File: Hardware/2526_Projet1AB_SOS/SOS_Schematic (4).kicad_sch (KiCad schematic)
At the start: 40 parts, among them J4 Conn_ST_STDC14, J5 USB_C_Receptacle_USB2.0_14P, SW1 SW_SPDT, U1 BU33SD5WG-TR, U2 STM32L476RGTx, U4 USBLC6-2SC6, Y1 13,56MHz, Y2 8MHz

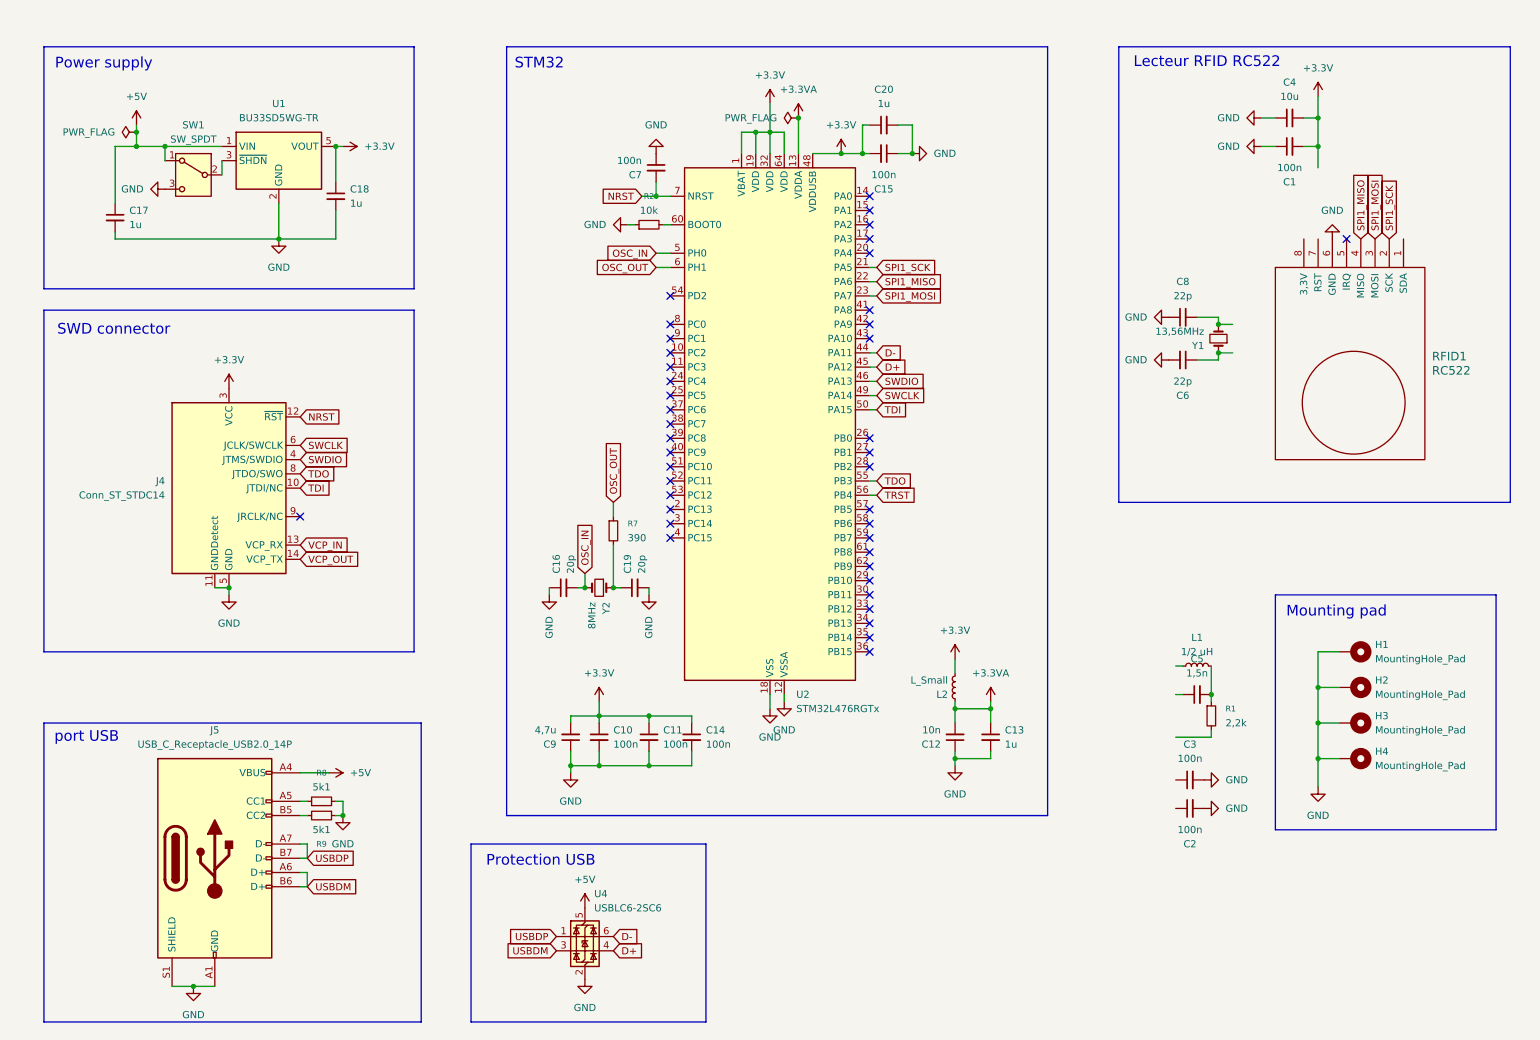
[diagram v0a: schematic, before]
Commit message: schematic v2
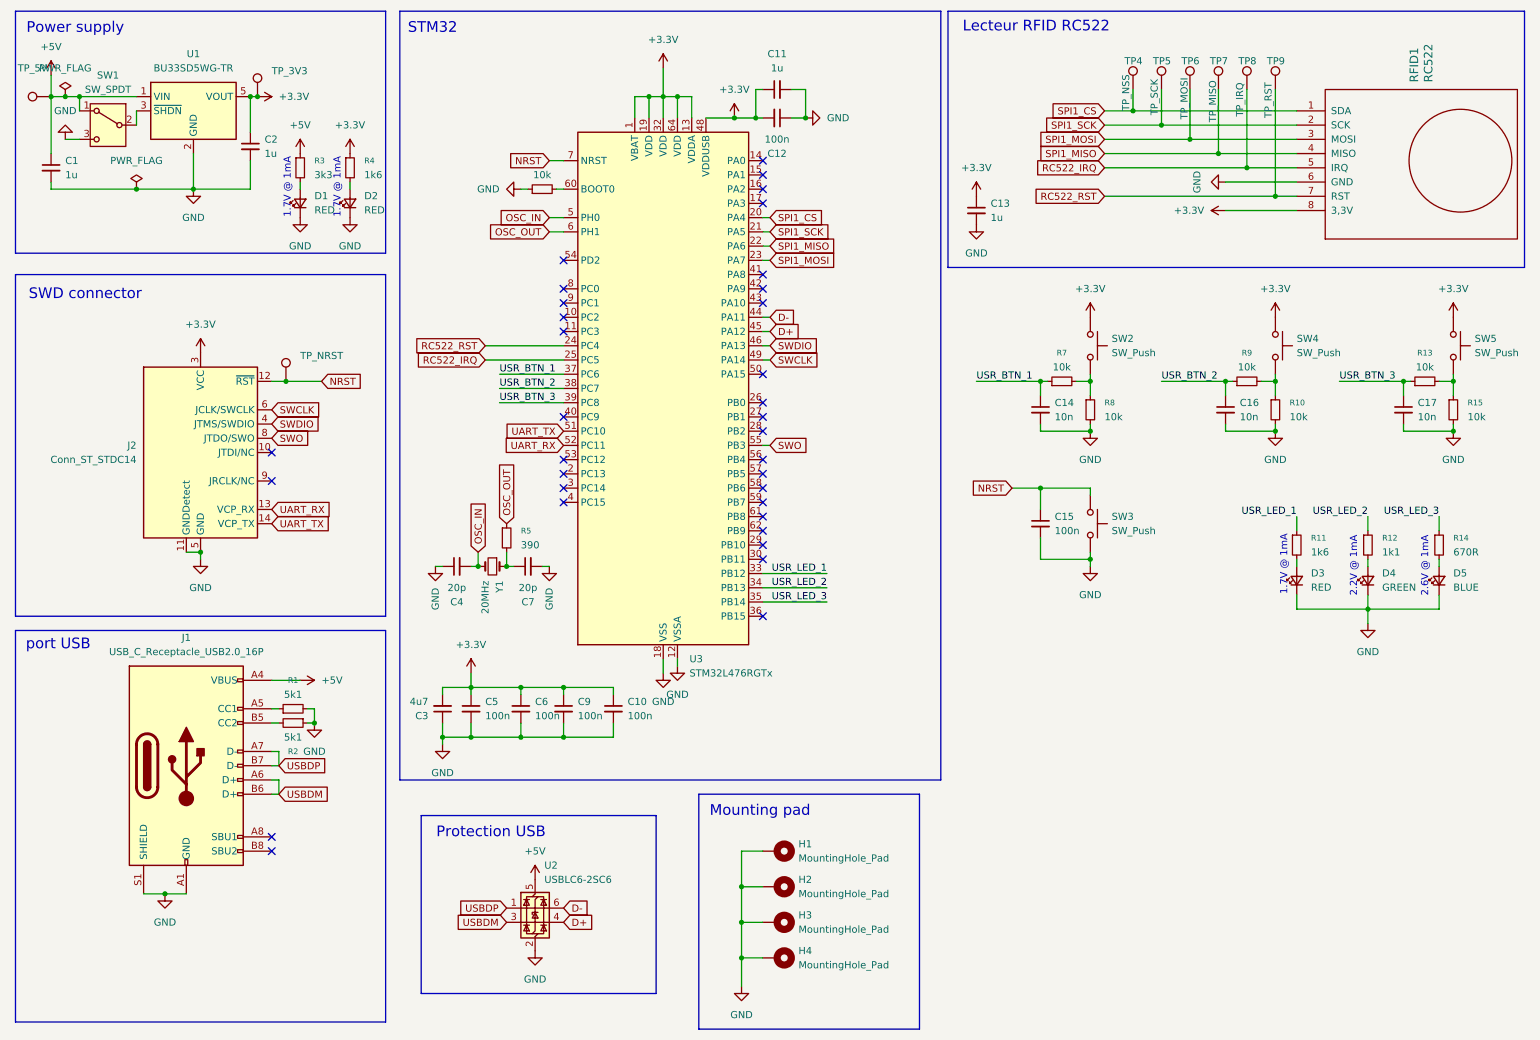
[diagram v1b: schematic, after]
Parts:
- removed C1, C2, C3, C7: 100n, Capacitor_SMD:C_0603_1608Metric_Pad1.08x0.95mm_HandSolder, symbol Device:C_Small
- removed C12: 10n, Capacitor_SMD:C_0603_1608Metric_Pad1.08x0.95mm_HandSolder, symbol Device:C_Small
- removed C4: 10u, Capacitor_SMD:C_0603_1608Metric_Pad1.08x0.95mm_HandSolder, symbol Device:C_Small
- removed C5: 1,5n, Capacitor_SMD:C_0603_1608Metric_Pad1.08x0.95mm_HandSolder, symbol Device:C_Small
- removed C6, C8: 22p, Capacitor_SMD:C_0603_1608Metric_Pad1.08x0.95mm_HandSolder, symbol Device:C_Small
- removed J5: USB_C_Receptacle_USB2.0_14P, symbol Connector:USB_C_Receptacle_USB2.0_14P
- removed L1: 1/2 uH, Inductor_SMD:L_0805_2012Metric_Pad1.05x1.20mm_HandSolder, symbol Device:L_Small
- removed L2: L_Small, Inductor_SMD:L_0805_2012Metric_Pad1.05x1.20mm_HandSolder, symbol Device:L_Small
- removed R1: 2,2k, Resistor_SMD:R_0805_2012Metric_Pad1.20x1.40mm_HandSolder, symbol Device:R_Small
- removed Y1: 13,56MHz, Crystal:Crystal_DS10_D1.0mm_L4.3mm_Vertical, symbol Device:Crystal_Small
- added C10, C15: 100n, Capacitor_SMD:C_0603_1608Metric, symbol Device:C_Small
- added C14, C16, C17: 10n, Capacitor_SMD:C_0603_1608Metric, symbol Device:C_Small
- added D1, D2, D3: RED, LED_SMD:LED_0603_1608Metric, symbol Device:LED_Small
- added D4: GREEN, LED_SMD:LED_0603_1608Metric, symbol Device:LED_Small
- added D5: BLUE, LED_SMD:LED_0603_1608Metric, symbol Device:LED_Small
- added J1: USB_C_Receptacle_USB2.0_16P, symbol Connector:USB_C_Receptacle_USB2.0_16P
- added R10, R13, R15, R7, R8, R9: 10k, Resistor_SMD:R_0603_1608Metric, symbol Device:R_Small
- added R11, R4: 1k6, Resistor_SMD:R_0603_1608Metric, symbol Device:R_Small
- added R12: 1k1, Resistor_SMD:R_0603_1608Metric, symbol Device:R_Small
- added R14: 670R, Resistor_SMD:R_0603_1608Metric, symbol Device:R_Small
- added R3: 3k3, Resistor_SMD:R_0603_1608Metric, symbol Device:R_Small
- added SW2, SW3, SW4, SW5: SW_Push, Button_Switch_SMD:SW_SPST_B3S-1000, symbol Switch:SW_Push
- added TP4: TP_NSS, TestPoint:TestPoint_Pad_D1.0mm, symbol Connector:TestPoint
- added TP5: TP_SCK, TestPoint:TestPoint_Pad_D1.0mm, symbol Connector:TestPoint
- added TP6: TP_MOSI, TestPoint:TestPoint_Pad_D1.0mm, symbol Connector:TestPoint
- added TP7: TP_MISO, TestPoint:TestPoint_Pad_D1.0mm, symbol Connector:TestPoint
- added TP8: TP_IRQ, TestPoint:TestPoint_Pad_D1.0mm, symbol Connector:TestPoint
- added TP9: TP_RST, TestPoint:TestPoint_Pad_D1.0mm, symbol Connector:TestPoint
- added TP_3V3: TP_3V3, TestPoint:TestPoint_Pad_D1.0mm, symbol Connector:TestPoint
- added TP_5V: TP_5V, TestPoint:TestPoint_Pad_D1.0mm, symbol Connector:TestPoint
- added TP_NRST: TP_NRST, TestPoint:TestPoint_Pad_D1.0mm, symbol Connector:TestPoint
- C1: renamed from C17; footprint Capacitor_SMD:C_0603_1608Metric_Pad1.08x0.95mm_HandSolder -> Capacitor_SMD:C_0603_1608Metric
- C11: renamed from C20; footprint Capacitor_SMD:C_0603_1608Metric_Pad1.08x0.95mm_HandSolder -> Capacitor_SMD:C_0603_1608Metric
- C12: renamed from C15; footprint Capacitor_SMD:C_0603_1608Metric_Pad1.08x0.95mm_HandSolder -> Capacitor_SMD:C_0603_1608Metric
- C13: footprint Capacitor_SMD:C_0603_1608Metric_Pad1.08x0.95mm_HandSolder -> Capacitor_SMD:C_0603_1608Metric
- C2: renamed from C18; footprint Capacitor_SMD:C_0603_1608Metric_Pad1.08x0.95mm_HandSolder -> Capacitor_SMD:C_0603_1608Metric
- C3: renamed from C9; value 4,7u -> 4u7; footprint Capacitor_SMD:C_0603_1608Metric_Pad1.08x0.95mm_HandSolder -> Capacitor_SMD:C_0603_1608Metric
- C4: renamed from C16; footprint Capacitor_SMD:C_0603_1608Metric_Pad1.08x0.95mm_HandSolder -> Capacitor_SMD:C_0603_1608Metric
- C5: renamed from C10; footprint Capacitor_SMD:C_0603_1608Metric_Pad1.08x0.95mm_HandSolder -> Capacitor_SMD:C_0603_1608Metric
- C6: renamed from C11; footprint Capacitor_SMD:C_0603_1608Metric_Pad1.08x0.95mm_HandSolder -> Capacitor_SMD:C_0603_1608Metric
- C7: renamed from C19; footprint Capacitor_SMD:C_0603_1608Metric_Pad1.08x0.95mm_HandSolder -> Capacitor_SMD:C_0603_1608Metric
- C9: renamed from C14; footprint Capacitor_SMD:C_0603_1608Metric_Pad1.08x0.95mm_HandSolder -> Capacitor_SMD:C_0603_1608Metric
- H1, H2, H3, H4: footprint MountingHole:MountingHole_3.2mm_M3_DIN965_Pad -> MountingHole:MountingHole_3.2mm_M3_Pad
- J2: renamed from J4; footprint Connector:Tag-Connect_TC2070-IDC-FP_2x07_P1.27mm_Vertical -> Connector_PinHeader_1.27mm:PinHeader_2x07_P1.27mm_Vertical_SMD
- R1: renamed from R8; footprint Resistor_SMD:R_0805_2012Metric_Pad1.20x1.40mm_HandSolder -> Resistor_SMD:R_0603_1608Metric
- R2: renamed from R9; footprint Resistor_SMD:R_0805_2012Metric_Pad1.20x1.40mm_HandSolder -> Resistor_SMD:R_0603_1608Metric
- R5: renamed from R7; footprint Resistor_SMD:R_0805_2012Metric_Pad1.20x1.40mm_HandSolder -> Resistor_SMD:R_0603_1608Metric
- R6: renamed from R2; footprint Resistor_SMD:R_0805_2012Metric_Pad1.20x1.40mm_HandSolder -> Resistor_SMD:R_0603_1608Metric
- RFID1: footprint (none) -> Connector_PinSocket_2.54mm:PinSocket_1x08_P2.54mm_Vertical
- Y1: renamed from Y2; value 8MHz -> 20MHz; footprint Crystal:Crystal_DS10_D1.0mm_L4.3mm_Vertical -> Crystal:Crystal_SMD_HC49-SD; MPN (none) -> ABLS-16.000MHZ-20-B-3-H-T
- renumbered U4 to U2, U2 to U3
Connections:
- net +3.3VA is gone; now on net +3.3V: C13.1, U3.13 (VDDA)
- net VCP_IN is gone; now on net UART_RX: J2.13 (VCP_RX)
- net VCP_OUT is gone; now on net UART_TX: J2.14 (VCP_TX)
- net +3.3V: now also RFID1.8 (3,3V), C10.1, R4.1, SW2.1, SW4.1, SW5.1, TP_3V3.1
- net +5V: now also J1.A4 (VBUS), J1.A9 (VBUS), J1.B4 (VBUS), J1.B9 (VBUS), R3.1, TP_5V.1
- net GND: now also C10.2, C14.2, C15.2, C16.2, C17.2, D1.1 (K), D2.1 (K), D3.1 (K), D4.1 (K), D5.1 (K), J1.A1 (GND), J1.A12 (GND), J1.B1 (GND), J1.B12 (GND), J1.S1 (SHIELD), R10.2, R15.2, R8.2, SW3.2
- net NRST: now also C15.1, SW3.1, TP_NRST.1
- net SPI1_MISO: now also TP7.1
- net SPI1_MOSI: now also TP6.1
- net SPI1_SCK: now also TP5.1
- net USBDM: now also J1.A6 (D+), J1.B6 (D+)
- net USBDP: now also J1.A7 (D-), J1.B7 (D-)
- net SPI1_CS: now reaches RFID1.1 (SDA)
- net SPI1_CS: now also U3.20 (PA4), TP4.1
- net RC522_IRQ: now reaches RFID1.5 (IRQ)
- net RC522_IRQ: now also U3.25 (PC5), TP8.1
- net RC522_RST: now reaches RFID1.7 (RST)
- net RC522_RST: now also U3.24 (PC4), TP9.1
- net USR_LED_1: now reaches U3.33 (PB12)
- net USR_LED_1: now also R11.1
- net USR_LED_2: now reaches U3.34 (PB13)
- net USR_LED_2: now also R12.1
- net USR_LED_3: now reaches U3.35 (PB14)
- net USR_LED_3: now also R14.1
- net USR_BTN_1: now reaches U3.37 (PC6)
- net USR_BTN_1: now also C14.1, R7.1
- net USR_BTN_2: now reaches U3.38 (PC7)
- net USR_BTN_2: now also C16.1, R9.1
- net USR_BTN_3: now reaches U3.39 (PC8)
- net USR_BTN_3: now also C17.1, R13.1
- net UART_TX: now reaches U3.51 (PC10)
- net UART_RX: now reaches U3.52 (PC11)
- net at R2.2: now also J1.B5 (CC2)
- net at R1.1: now also J1.A5 (CC1)
- net TDI: no longer names the net of J2.10 (JTDI/NC)
- net TDI: no longer U3.50 (PA15)
- net TDO renamed SWO
- net TRST: no longer names the net of U3.56 (PB4)
- new net: R7.2, R8.1, SW2.2
- new net: D4.2 (A), R12.2
- new net: R13.2, R15.1, SW5.2
- new net: D3.2 (A), R11.2
- new net: R10.1, R9.2, SW4.2
- new net: D1.2 (A), R3.2
- new net: D5.2 (A), R14.2
- new net: D2.2 (A), R4.2
- no-connect marks 41 -> 34
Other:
- note added: "1.7V @ 1mA"
- note added: "2.2V @ 1mA"
- note added: "2.6V @ 1mA"
- moved on the sheet: C1, C11, C12, C2, C3, C4, C5, C6, C7, C9, H1, H2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
